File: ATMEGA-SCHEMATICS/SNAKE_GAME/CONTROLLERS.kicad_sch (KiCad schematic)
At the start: 18 parts, among them J12 USB_ASP, J13 UART_TERM, J14 BUTTONS, J15 PCF_SCREEN, J16 GROUND, J17 JOYSTICK, J18 VCC, J2 GRID

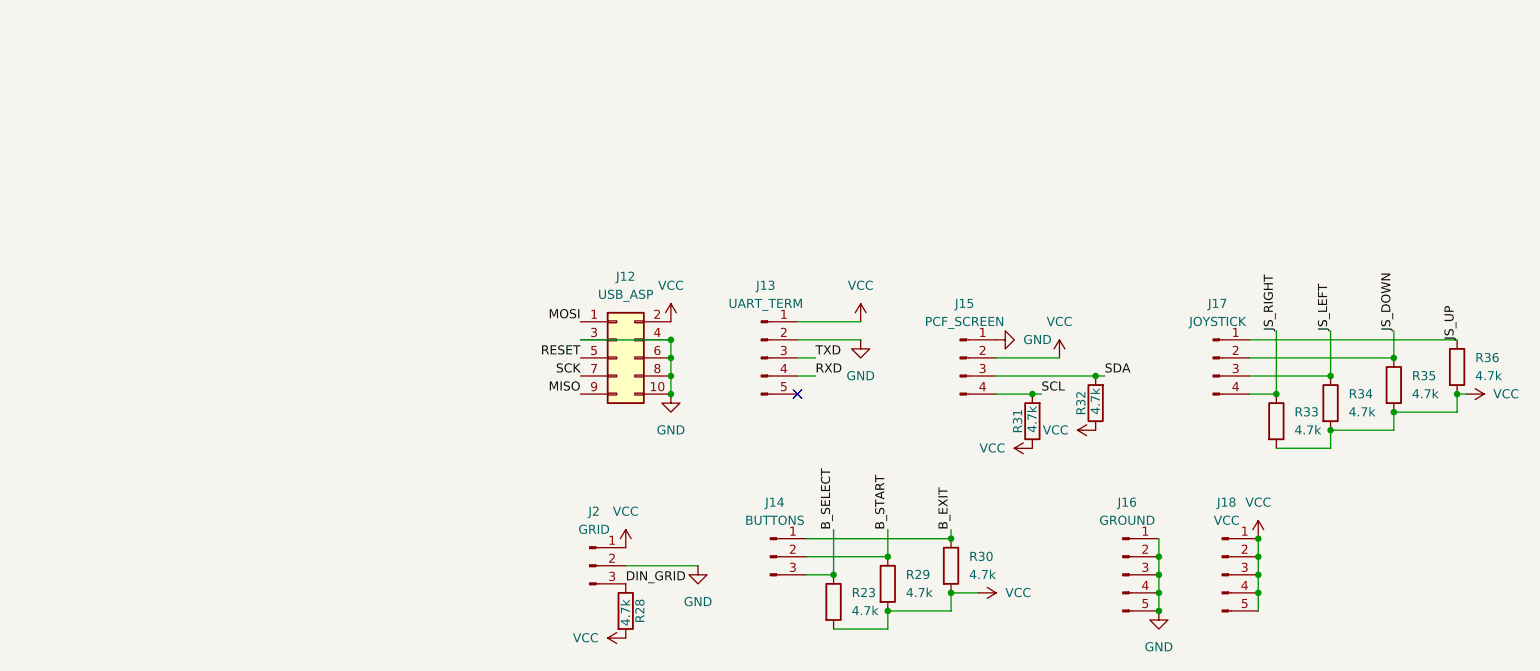
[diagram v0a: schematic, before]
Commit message: .
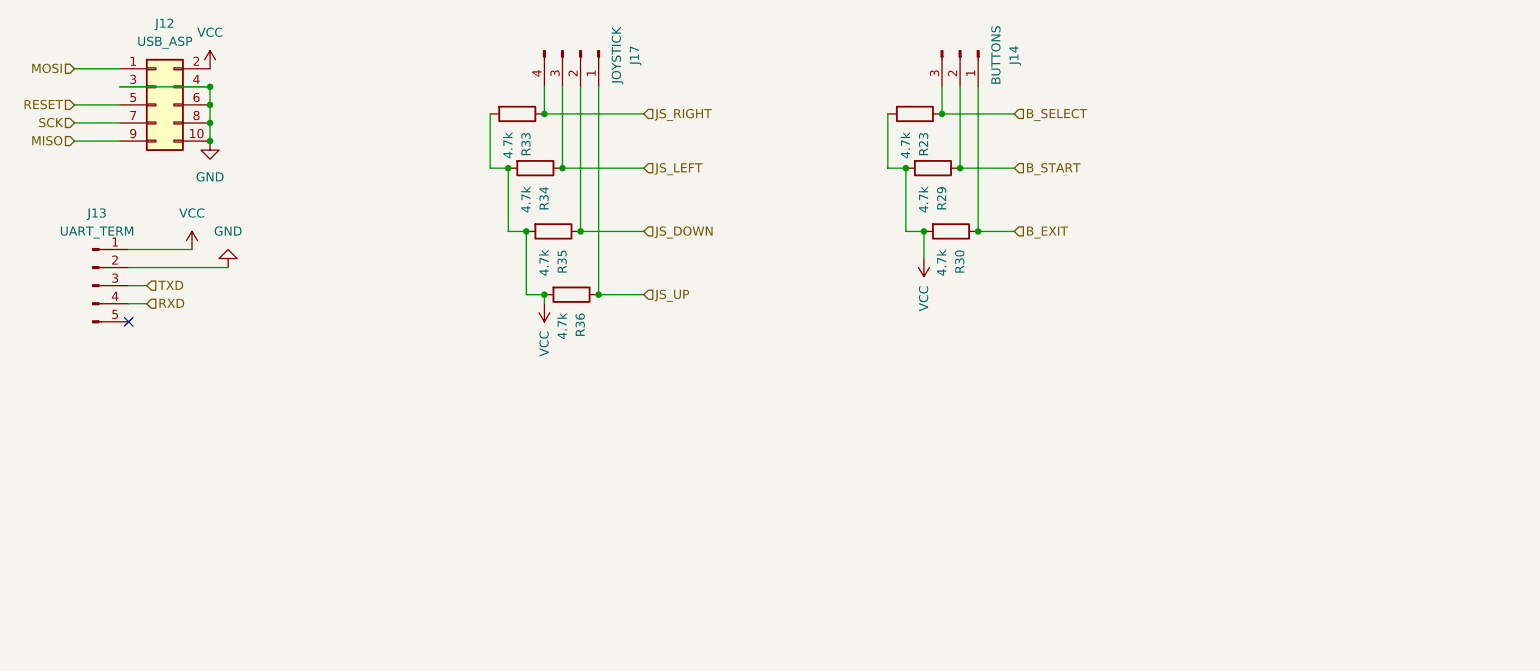
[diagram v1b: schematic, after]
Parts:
- removed J15: PCF_SCREEN, TerminalBlock:TerminalBlock_MaiXu_MX126-5.0-04P_1x04_P5.00mm, symbol Connector:Conn_01x04_Pin
- removed J16: GROUND, TerminalBlock:TerminalBlock_MaiXu_MX126-5.0-04P_1x04_P5.00mm, symbol Connector:Conn_01x05_Pin
- removed J18: VCC, TerminalBlock:TerminalBlock_MaiXu_MX126-5.0-04P_1x04_P5.00mm, symbol Connector:Conn_01x05_Pin
- removed J2: GRID, TerminalBlock:TerminalBlock_MaiXu_MX126-5.0-03P_1x03_P5.00mm, symbol Connector:Conn_01x03_Pin
- removed R28, R31, R32: 4.7k, Resistor_THT:R_Axial_DIN0207_L6.3mm_D2.5mm_P10.16mm_Horizontal, symbol Device:R
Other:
- moved on the sheet: J12, J13, J14, J17, R23, R29, R30, R33, R34, R35, R36
